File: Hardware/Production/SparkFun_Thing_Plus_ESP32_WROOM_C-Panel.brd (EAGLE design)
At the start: 106.7 x 207 mm, 1314 parts, among them J10 THING_PLUS_LOGICAL, J11 QWIIC_RA, J14 MICRO-SDFRICTION, J15 THING_PLUS_LOGICAL, J16 QWIIC_RA, J19 MICRO-SDFRICTION, J2 MICRO-SDFRICTION, J20 THING_PLUS_LOGICAL, J21 QWIIC_RA, J24 MICRO-SDFRICTION, J25 THING_PLUS_LOGICAL, J26 QWIIC_RA, J29 MICRO-SDFRICTION, J3 QWIIC_RA, J30 THING_PLUS_LOGICAL, J31 QWIIC_RA, J34 MICRO-SDFRICTION, J35 THING_PLUS_LOGICAL, J36 QWIIC_RA, J39 MICRO-SDFRICTION, J40 THING_PLUS_LOGICAL, J41 QWIIC_RA, J44 MICRO-SDFRICTION, J45 THING_PLUS_LOGICAL, J46 QWIIC_RA, J49 MICRO-SDFRICTION, J5 THING_PLUS_LOGICAL, J50 THING_PLUS_LOGICAL, J51 QWIIC_RA, J54 MICRO-SDFRICTION, J55 THING_PLUS_LOGICAL, J56 QWIIC_RA, J59 MICRO-SDFRICTION, J6 QWIIC_RA, J60 THING_PLUS_LOGICAL, J9 MICRO-SDFRICTION, Q1 MBT3904DW1T1, Q10 20V/4.2A/52mΩ/1.4W, Q11 MBT3904DW1T1, Q12 20V/4.2A/52mΩ/1.4W, Q13 MBT3904DW1T1, Q14 20V/4.2A/52mΩ/1.4W, Q15 MBT3904DW1T1, Q16 20V/4.2A/52mΩ/1.4W, Q17 MBT3904DW1T1, Q18 20V/4.2A/52mΩ/1.4W, Q19 MBT3904DW1T1, Q2 MBT3904DW1T1, Q20 20V/4.2A/52mΩ/1.4W, Q21 MBT3904DW1T1, Q22 20V/4.2A/52mΩ/1.4W, Q23 MBT3904DW1T1, Q24 20V/4.2A/52mΩ/1.4W, Q3 20V/4.2A/52mΩ/1.4W, Q4 20V/4.2A/52mΩ/1.4W, Q5 MBT3904DW1T1, Q6 20V/4.2A/52mΩ/1.4W, Q7 MBT3904DW1T1, Q8 20V/4.2A/52mΩ/1.4W, Q9 MBT3904DW1T1, U1 MCP73831, U10 XC6222B331MR-G, U11 XC6222B331MR-G, U12 ESP-WROOM-3232D-NARROW, U13 MCP73831, U14 CH340C, U15 MAX17048, U16 XC6222B331MR-G, U17 XC6222B331MR-G, U18 ESP-WROOM-3232D-NARROW, U19 MCP73831, U2 ESP-WROOM-3232D-NARROW, U20 CH340C, U21 MAX17048, U22 XC6222B331MR-G, U23 XC6222B331MR-G, U24 ESP-WROOM-3232D-NARROW, U25 MCP73831, U26 CH340C, U27 MAX17048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

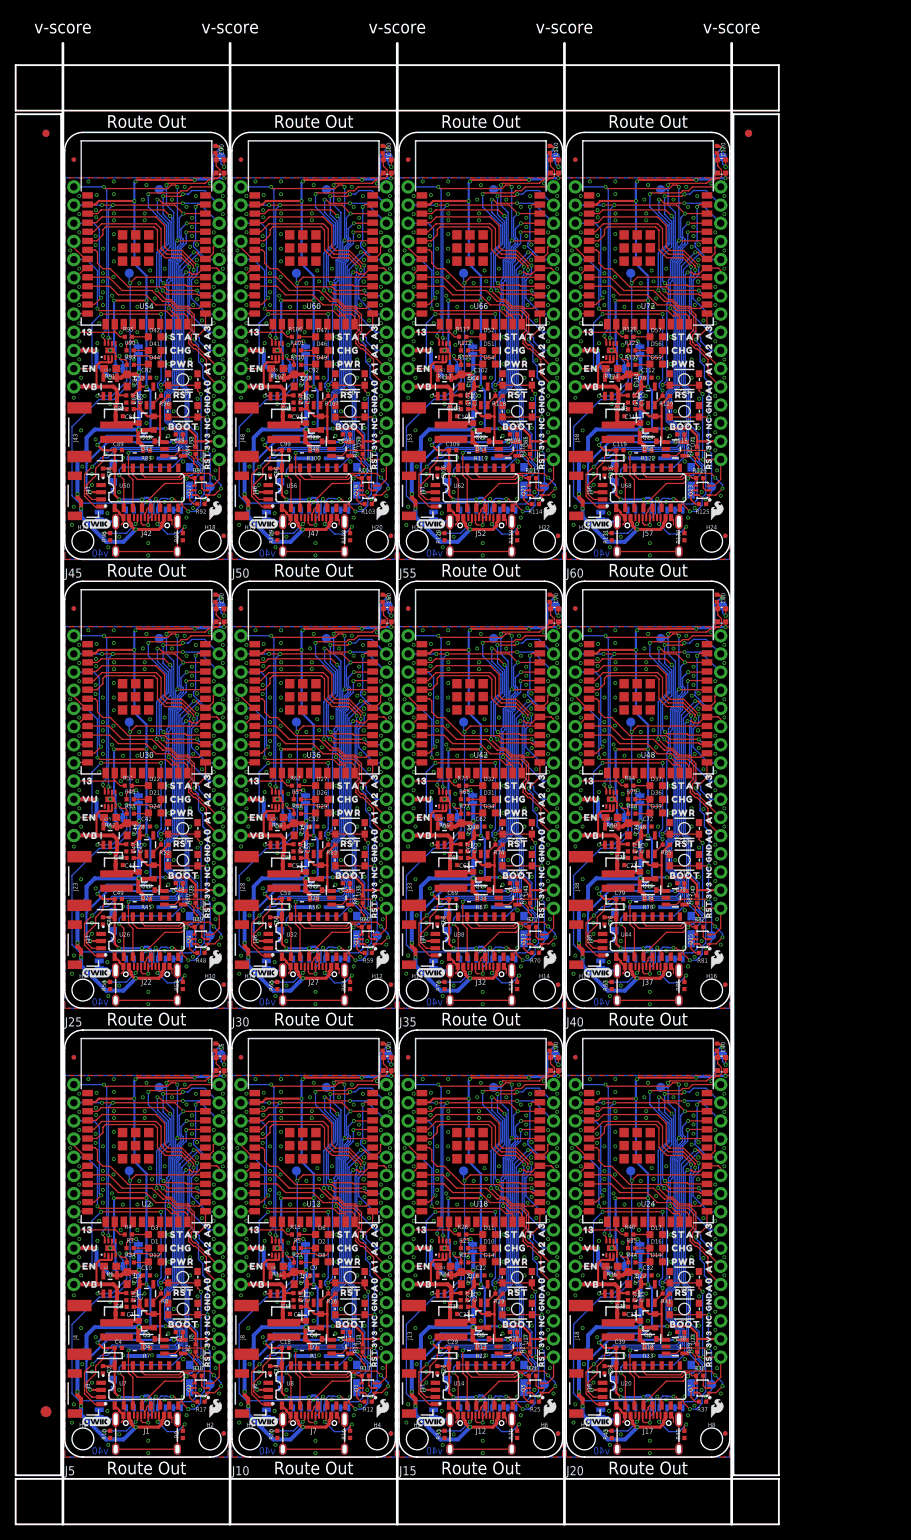
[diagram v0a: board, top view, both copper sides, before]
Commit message: Updated panel
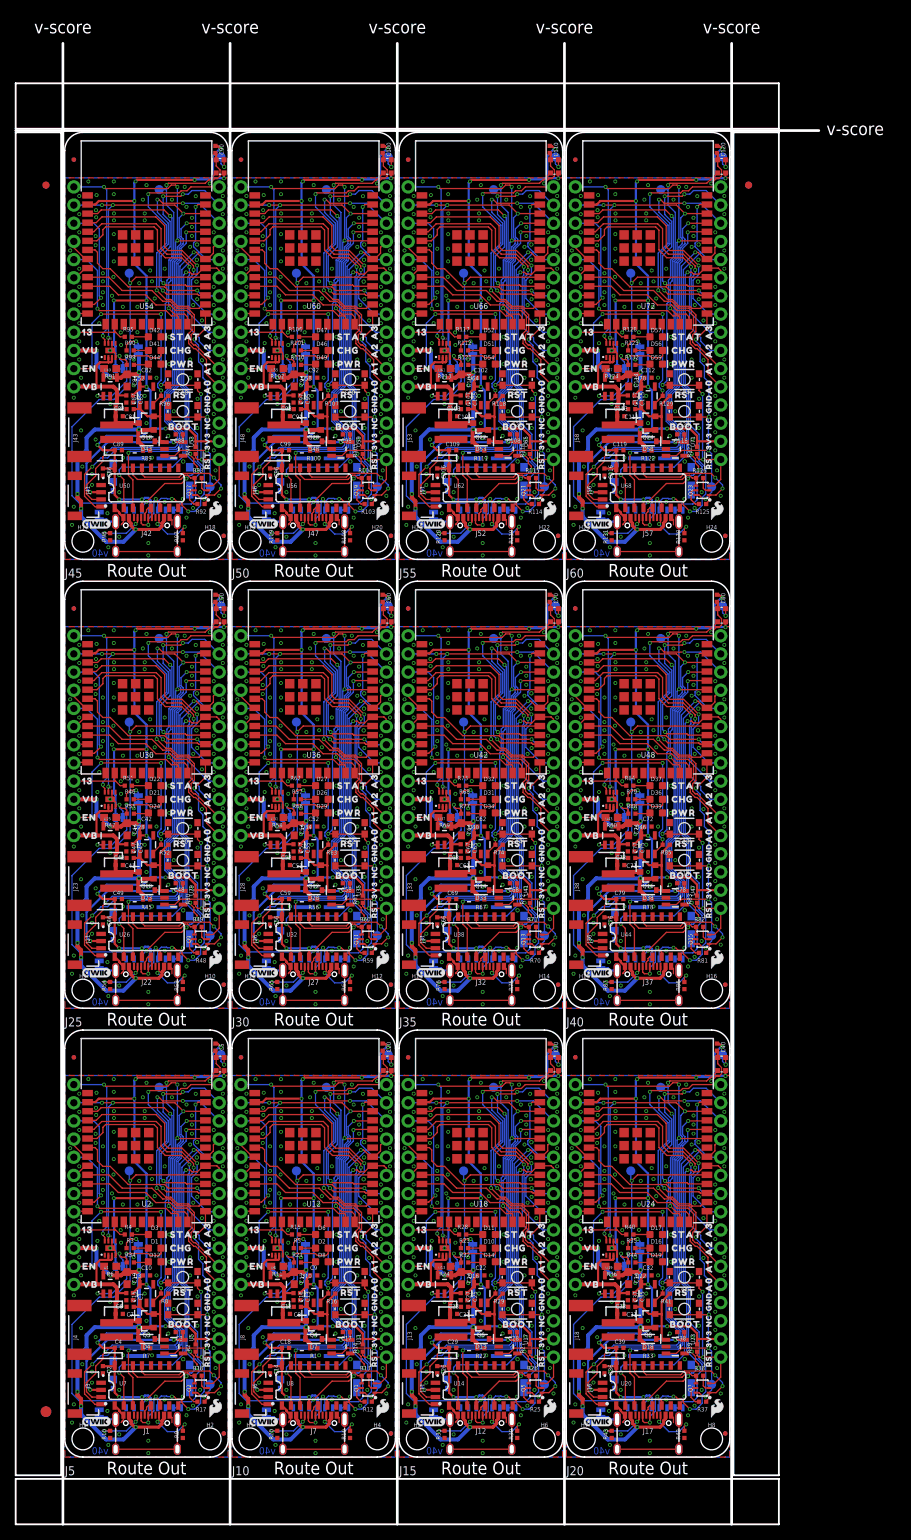
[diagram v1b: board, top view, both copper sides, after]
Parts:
- moved E$1 7.24 mm to (-2.62, 177.8)
- moved E$2 7.24 mm to (-2.62, 177.8)
- moved E$3 7.24 mm to (95.6, 177.8)
- moved E$4 7.24 mm to (95.6, 177.8)
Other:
- board size 106.7 x 207 mm -> 112.3 x 207 mm
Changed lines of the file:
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@@
 <rectangle x1="7.7724" y1="149.4028" x2="7.9502" y2="149.9108" layer="41"/>
 <text x="11.43" y="123.952" size="1.778" layer="20" ratio="15" align="center">Route Out</text>
-<text x="11.43" y="186.69" size="1.778" layer="20" ratio="15" align="center">Route Out</text>
 <wire x1="46.228" y1="128.016" x2="46.228" y2="182.626" width="0.2032" layer="20"/>
 <wire x1="46.228" y1="182.626" x2="43.688" y2="185.166" width="0.2032" layer="20" curve="90"/>
@@
 <rectangle x1="31.1404" y1="149.4028" x2="31.3182" y2="149.9108" layer="41"/>
 <text x="34.798" y="123.952" size="1.778" layer="20" ratio="15" align="center">Route Out</text>
-<text x="34.798" y="186.69" size="1.778" layer="20" ratio="15" align="center">Route Out</text>
 <wire x1="69.596" y1="128.016" x2="69.596" y2="182.626" width="0.2032" layer="20"/>
 <wire x1="69.596" y1="182.626" x2="67.056" y2="185.166" width="0.2032" layer="20" curve="90"/>
@@
 <rectangle x1="54.5084" y1="149.4028" x2="54.6862" y2="149.9108" layer="41"/>
 <text x="58.166" y="123.952" size="1.778" layer="20" ratio="15" align="center">Route Out</text>
-<text x="58.166" y="186.69" size="1.778" layer="20" ratio="15" align="center">Route Out</text>
 <wire x1="92.964" y1="128.016" x2="92.964" y2="182.626" width="0.2032" layer="20"/>
 <wire x1="92.964" y1="182.626" x2="90.424" y2="185.166" width="0.2032" layer="20" curve="90"/>
@@
 <rectangle x1="77.8764" y1="149.4028" x2="78.0542" y2="149.9108" layer="41"/>
 <text x="81.534" y="123.952" size="1.778" layer="20" ratio="15" align="center">Route Out</text>
-<text x="81.534" y="186.69" size="1.778" layer="20" ratio="15" align="center">Route Out</text>
 <wire x1="-0.254" y1="-9.398" x2="-0.254" y2="197.612" width="0.381" layer="46"/>
 <text x="-0.254" y="199.898" size="1.778" layer="46" ratio="15" align="center">v-score</text>
@@
 <wire x1="99.822" y1="-9.398" x2="-6.858" y2="-9.398" width="0.254" layer="20"/>
 <wire x1="-6.858" y1="-9.398" x2="-6.858" y2="-3.048" width="0.254" layer="20"/>
-<wire x1="93.472" y1="187.706" x2="99.822" y2="187.706" width="0.254" layer="20"/>
-<wire x1="99.822" y1="187.706" x2="99.822" y2="-2.54" width="0.254" layer="20"/>
+<wire x1="93.472" y1="185.166" x2="99.822" y2="185.166" width="0.254" layer="20"/>
+<wire x1="99.822" y1="185.166" x2="99.822" y2="-2.54" width="0.254" layer="20"/>
 <wire x1="99.822" y1="-2.54" x2="93.472" y2="-2.54" width="0.254" layer="20"/>
-<wire x1="93.472" y1="-2.54" x2="93.472" y2="187.706" width="0.254" layer="20"/>
-<wire x1="-6.858" y1="194.564" x2="99.822" y2="194.564" width="0.254" layer="20"/>
-<wire x1="99.822" y1="194.564" x2="99.822" y2="188.214" width="0.254" layer="20"/>
-<wire x1="99.822" y1="188.214" x2="-6.858" y2="188.214" width="0.254" layer="20"/>
-<wire x1="-6.858" y1="188.214" x2="-6.858" y2="194.564" width="0.254" layer="20"/>
-<wire x1="-6.858" y1="187.706" x2="-0.508" y2="187.706" width="0.254" layer="20"/>
-<wire x1="-0.508" y1="187.706" x2="-0.508" y2="-2.54" width="0.254" layer="20"/>
+<wire x1="93.472" y1="-2.54" x2="93.472" y2="185.166" width="0.254" layer="20"/>
+<wire x1="-6.858" y1="192.024" x2="99.822" y2="192.024" width="0.254" layer="20"/>
+<wire x1="99.822" y1="192.024" x2="99.822" y2="185.674" width="0.254" layer="20"/>
+<wire x1="99.822" y1="185.674" x2="-6.858" y2="185.674" width="0.254" layer="20"/>
+<wire x1="-6.858" y1="185.674" x2="-6.858" y2="192.024" width="0.254" layer="20"/>
+<wire x1="-6.858" y1="185.166" x2="-0.508" y2="185.166" width="0.254" layer="20"/>
+<wire x1="-0.508" y1="185.166" x2="-0.508" y2="-2.54" width="0.254" layer="20"/>
 <wire x1="-0.508" y1="-2.54" x2="-6.858" y2="-2.54" width="0.254" layer="20"/>
-<wire x1="-6.858" y1="-2.54" x2="-6.858" y2="187.706" width="0.254" layer="20"/>
+<wire x1="-6.858" y1="-2.54" x2="-6.858" y2="185.166" width="0.254" layer="20"/>
+<wire x1="-6.858" y1="185.42" x2="105.41" y2="185.42" width="0.381" layer="46"/>
+<text x="110.49" y="185.674" size="1.778" layer="46" ratio="15" align="center">v-score</text>
 </plain>
 <attributes>
@@
 <element name="U$623" library="SparkFun-Aesthetics" package="SFE_LOGO_FLAME_.1" value="" x="91.186" y="132.334" smashed="yes"/>
 <element name="U$624" library="output" package="#SHLD#0" value="" x="74.93" y="132.4102" smashed="yes" rot="MR90"/>
-<element name="E$1" library="SparkFun-Aesthetics" package="FIDUCIAL-1X2" value="" x="-2.62381875" y="185.039" smashed="yes"/>
-<element name="E$2" library="SparkFun-Aesthetics" package="FIDUCIAL-1X2" value="" x="-2.62381875" y="185.039" smashed="yes" rot="MR0"/>
-<element name="E$3" library="SparkFun-Aesthetics" package="FIDUCIAL-1X2" value="" x="95.58781875" y="185.039" smashed="yes"/>
-<element name="E$4" library="SparkFun-Aesthetics" package="FIDUCIAL-1X2" value="" x="95.58781875" y="185.039" smashed="yes" rot="MR0"/>
+<element name="E$1" library="SparkFun-Aesthetics" package="FIDUCIAL-1X2" value="" x="-2.62381875" y="177.8" smashed="yes"/>
+<element name="E$2" library="SparkFun-Aesthetics" package="FIDUCIAL-1X2" value="" x="-2.62381875" y="177.8" smashed="yes" rot="MR0"/>
+<element name="E$3" library="SparkFun-Aesthetics" package="FIDUCIAL-1X2" value="" x="95.58781875" y="177.8" smashed="yes"/>
+<element name="E$4" library="SparkFun-Aesthetics" package="FIDUCIAL-1X2" value="" x="95.58781875" y="177.8" smashed="yes" rot="MR0"/>
 <element name="E$5" library="SparkFun-Retired" package="FIDUCIAL-1.5X3" value="" x="-2.62381875" y="6.35" smashed="yes"/>
 <element name="E$6" library="SparkFun-Retired" package="FIDUCIAL-1.5X3" value="" x="-2.62381875" y="6.35" smashed="yes" rot="MR0"/>
